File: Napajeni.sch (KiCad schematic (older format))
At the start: 8 parts, among them Q1 BS250, Q4 BS250, Q5 NTR2101P, SW2 SW_MEC_5G

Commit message: Mosfet
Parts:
- removed Q5: NTR2101P, Package_TO_SOT_SMD:SOT-23, symbol Transistor_FET:NTR2101P
- added Q2: 2N7000, Package_TO_SOT_THT:TO-92_Inline, symbol Transistor_FET:2N7000
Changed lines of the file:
@@
 	1    0    0    -1
-$EndComp
-$Comp
-L Transistor_FET:NTR2101P Q5
-U 1 1 601B9875
-P 7300 3100
-F 0 "Q5" V 7500 3050 50  0000 L CNN
-F 1 "NTR2101P" V 7500 2650 50  0000 L CNN
-F 2 "Package_TO_SOT_SMD:SOT-23" H 7500 3025 50  0001 L CIN
-F 3 "http://www.onsemi.com/pub/Collateral/NTR2101P-D.PDF" H 7300 3100 50  0001 L CNN
-	1    7300 3100
-	-1   0    0    -1
 $EndComp
 Wire Wire Line
@@
 Wire Wire Line
 	7200 2500 7200 2900
+$Comp
+L Transistor_FET:2N7000 Q2
+U 1 1 60247708
+P 7300 3100
+F 0 "Q2" H 7505 3054 50  0000 L CNN
+F 1 "2N7000" H 7505 3145 50  0000 L CNN
+F 2 "Package_TO_SOT_THT:TO-92_Inline" H 7500 3025 50  0001 L CIN
+F 3 "https://www.onsemi.com/pub/Collateral/NDS7002A-D.PDF" H 7300 3100 50  0001 L CNN
+	1    7300 3100
+	-1   0    0    1
+$EndComp
 $EndSCHEMATC

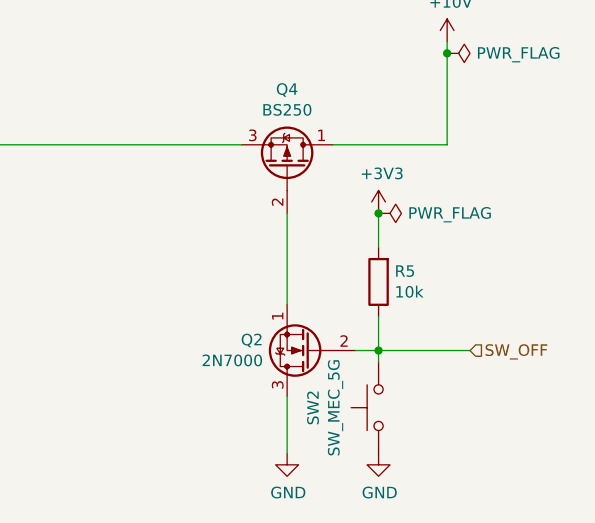
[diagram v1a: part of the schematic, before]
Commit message: Jirka upravy
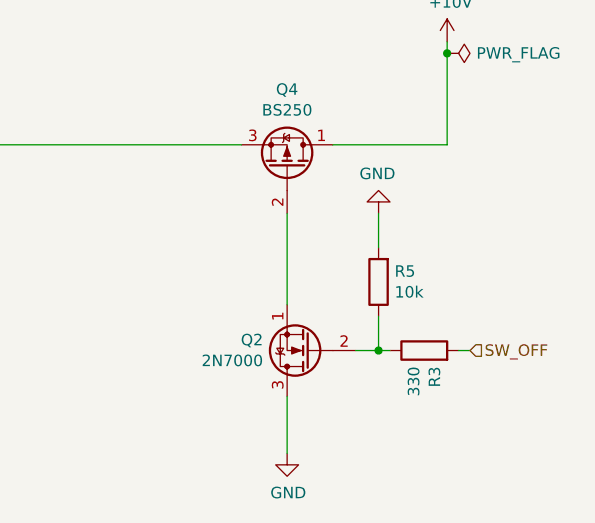
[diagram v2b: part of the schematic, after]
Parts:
- removed SW2: SW_MEC_5G, symbol Switch:SW_MEC_5G
- added R3: 330, symbol Device:R
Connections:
- net +3V3 is gone; now on net GND: R5.2
- net SW_OFF: now also R3.2; no longer Q2.2 (G), R5.1
- new net: Q2.2 (G), R3.1, R5.1
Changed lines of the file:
@@
 L power:GND #PWR011
 U 1 1 601BC6CA
-P 7600 3550
-F 0 "#PWR011" H 7600 3300 50  0001 C CNN
-F 1 "GND" H 7605 3377 50  0000 C CNN
-F 2 "" H 7600 3550 50  0001 C CNN
-F 3 "" H 7600 3550 50  0001 C CNN
-	1    7600 3550
-	1    0    0    -1
-$EndComp
-$Comp
-L Switch:SW_MEC_5G SW2
-U 1 1 601BC87E
-P 7600 3350
-F 0 "SW2" H 7600 3635 50  0000 C CNN
-F 1 "SW_MEC_5G" H 7600 3544 50  0000 C CNN
-F 2 "" H 7600 3550 50  0001 C CNN
-F 3 "http://www.apem.com/int/index.php?controller=attachment&id_attachment=488" H 7600 3550 50  0001 C CNN
-	1    7600 3350
-	0    -1   -1   0
+P 7600 2500
+F 0 "#PWR011" H 7600 2250 50  0001 C CNN
+F 1 "GND" H 7605 2327 50  0000 C CNN
+F 2 "" H 7600 2500 50  0001 C CNN
+F 3 "" H 7600 2500 50  0001 C CNN
+	1    7600 2500
+	-1   0    0    1
 $EndComp
 Wire Wire Line
 	7500 3100 7600 3100
-Wire Wire Line
-	7600 3100 7600 3150
 Wire Wire Line
 	7600 3100 7600 2950
@@
 SW_OFF
 Wire Wire Line
-	8000 3100 7600 3100
+	8000 3100 7950 3100
 $Comp
 L power:PWR_FLAG #FLG0101
@@
 Wire Wire Line
 	7600 2650 7600 2500
-$Comp
-L power:+3V3 #PWR0103
-U 1 1 601A3014
-P 7600 2500
-F 0 "#PWR0103" H 7600 2350 50  0001 C CNN
-F 1 "+3V3" H 7615 2673 50  0000 C CNN
-F 2 "" H 7600 2500 50  0001 C CNN
-F 3 "" H 7600 2500 50  0001 C CNN
-	1    7600 2500
-	1    0    0    -1
-$EndComp
-$Comp
-L power:PWR_FLAG #FLG0103
-U 1 1 601B3EBD
-P 7600 2500
-F 0 "#FLG0103" H 7600 2575 50  0001 C CNN
-F 1 "PWR_FLAG" V 7600 2628 50  0000 L CNN
-F 2 "" H 7600 2500 50  0001 C CNN
-F 3 "~" H 7600 2500 50  0001 C CNN
-	1    7600 2500
-	0    1    1    0
-$EndComp
-Connection ~ 7600 2500
 Wire Wire Line
 	4450 2500 5250 2500
@@
 	-1   0    0    1
 $EndComp
+$Comp
+L Device:R R3
+U 1 1 602489A5
+P 7800 3100
+F 0 "R3" H 7730 3054 50  0000 R CNN
+F 1 "330" H 7730 3145 50  0000 R CNN
+F 2 "" V 7730 3100 50  0001 C CNN
+F 3 "~" H 7800 3100 50  0001 C CNN
+	1    7800 3100
+	0    -1   -1   0
+$EndComp
+Wire Wire Line
+	7650 3100 7600 3100
 $EndSCHEMATC

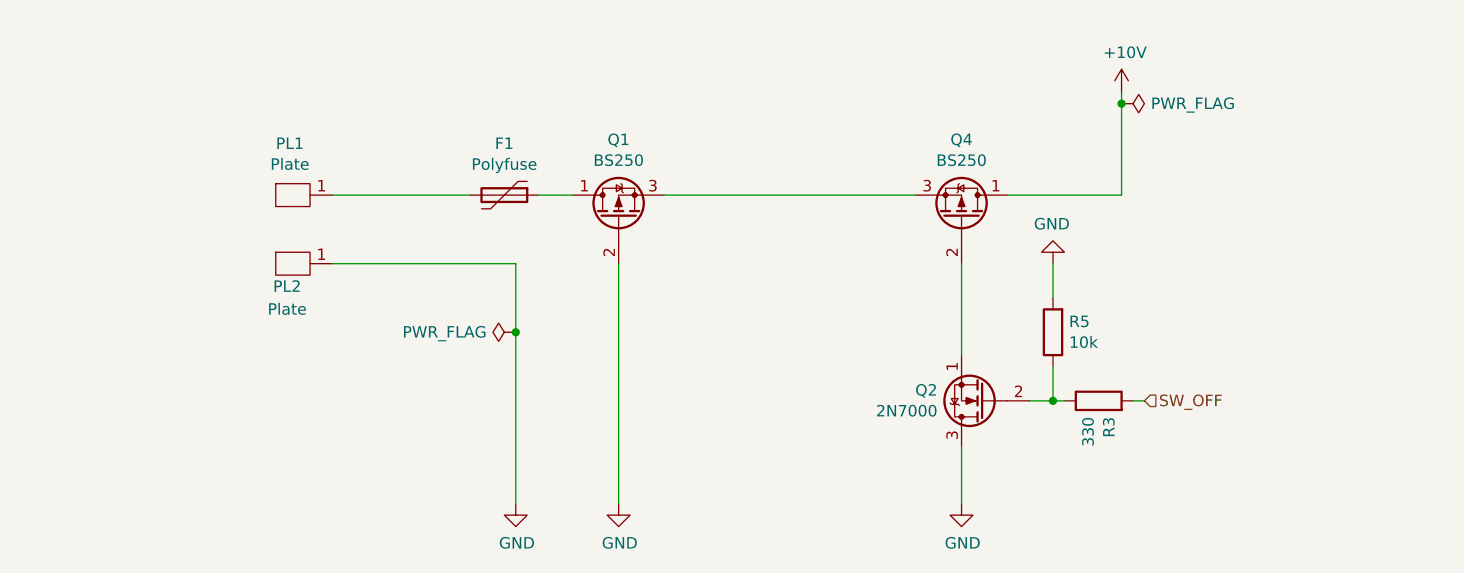
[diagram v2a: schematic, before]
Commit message: Hotové schéma
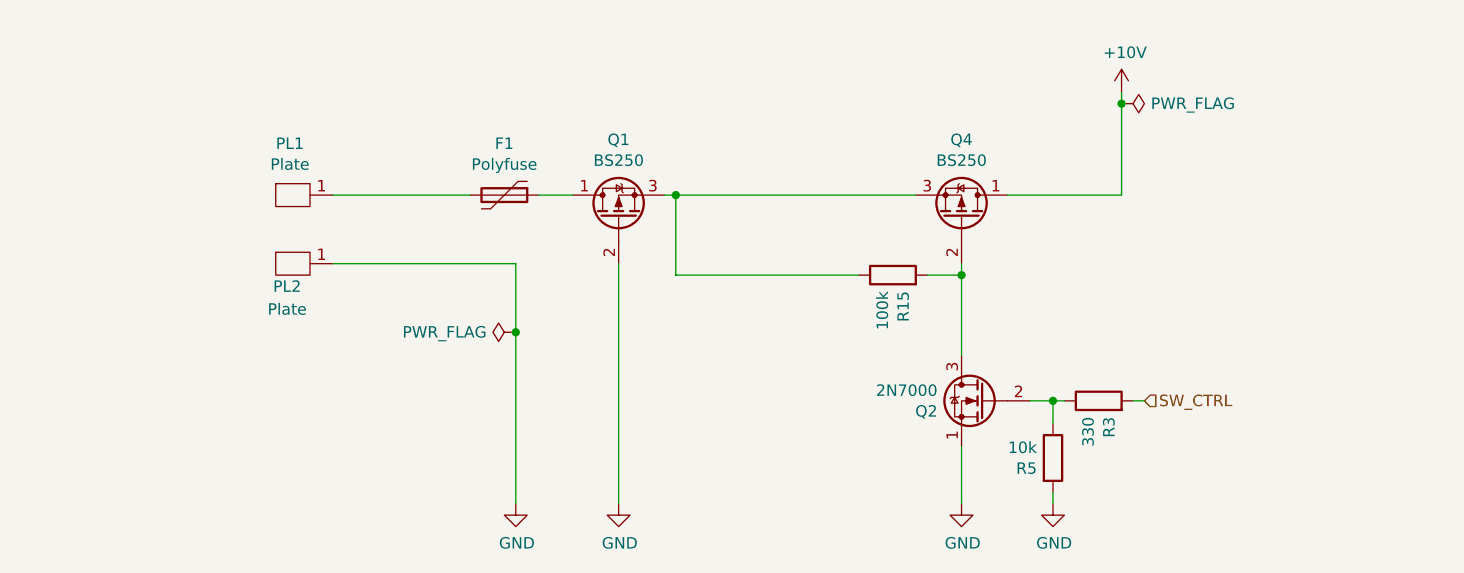
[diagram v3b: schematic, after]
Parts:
- added R15: 100k, Resistor_SMD:R_0805_2012Metric_Pad1.20x1.40mm_HandSolder, symbol Device:R
- Q2: LCSC (none) -> C8545
- R3: footprint (none) -> Resistor_SMD:R_0805_2012Metric_Pad1.20x1.40mm_HandSolder; LCSC (none) -> C17617
- R5: footprint (none) -> Resistor_SMD:R_0805_2012Metric_Pad1.20x1.40mm_HandSolder; LCSC (none) -> C17414
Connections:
- net GND: now also Q2.1 (S); no longer Q2.3 (D)
- net at Q1.3 (S), Q4.3 (S): now also R15.1
- net at Q4.2 (G): now also Q2.3 (D), R15.2; no longer Q2.1 (S)
- net SW_OFF renamed SW_CTRL
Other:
- moved on the sheet: R5
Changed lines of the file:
@@
 L Device:R R5
 U 1 1 601BBFD0
-P 7600 2800
-F 0 "R5" H 7530 2754 50  0000 R CNN
-F 1 "10k" H 7530 2845 50  0000 R CNN
-F 2 "" V 7530 2800 50  0001 C CNN
-F 3 "~" H 7600 2800 50  0001 C CNN
-	1    7600 2800
-	-1   0    0    1
+P 7600 3350
+F 0 "R5" H 7530 3304 50  0000 R CNN
+F 1 "10k" H 7530 3395 50  0000 R CNN
+F 2 "Resistor_SMD:R_0805_2012Metric_Pad1.20x1.40mm_HandSolder" V 7530 3350 50  0001 C CNN
+F 3 "~" H 7600 3350 50  0001 C CNN
+F 4 "C17414	" H 7600 3350 50  0001 C CNN "LCSC"
+	1    7600 3350
+	1    0    0    -1
 $EndComp
 $Comp
 L power:GND #PWR011
 U 1 1 601BC6CA
-P 7600 2500
-F 0 "#PWR011" H 7600 2250 50  0001 C CNN
-F 1 "GND" H 7605 2327 50  0000 C CNN
-F 2 "" H 7600 2500 50  0001 C CNN
-F 3 "" H 7600 2500 50  0001 C CNN
-	1    7600 2500
-	-1   0    0    1
+P 7600 3550
+F 0 "#PWR011" H 7600 3300 50  0001 C CNN
+F 1 "GND" H 7605 3377 50  0000 C CNN
+F 2 "" H 7600 3550 50  0001 C CNN
+F 3 "" H 7600 3550 50  0001 C CNN
+	1    7600 3550
+	1    0    0    -1
 $EndComp
-Wire Wire Line
-	7500 3100 7600 3100
-Wire Wire Line
-	7600 3100 7600 2950
-Connection ~ 7600 3100
 Text HLabel 8000 3100 2    50   Input ~ 0
-SW_OFF
+SW_CTRL
 Wire Wire Line
 	8000 3100 7950 3100
@@
 $EndComp
 Wire Wire Line
-	7600 2650 7600 2500
-Wire Wire Line
 	4450 2500 5250 2500
 $Comp
@@
 F 3 "" H 4250 2200 50  0001 C CNN
 	1    4250 2200
-	0    1    1    0
-$EndComp
-$Comp
-L Základní-deska-II-rescue:Plate-Tmc2209BreakoutBoard PL2
-U 1 1 601FAA1F
-P 4250 2500
-F 0 "PL2" V 4350 2500 50  0000 C CNN
-F 1 "Plate" V 4450 2500 50  0000 C CNN
-F 2 "" H 4250 2500 50  0001 C CNN
-F 3 "" H 4250 2500 50  0001 C CNN
-	1    4250 2500
 	0    1    1    0
 $EndComp
@@
 $EndComp
 Wire Wire Line
-	5900 2200 7000 2200
+	5900 2200 5950 2200
 Wire Wire Line
-	7200 2500 7200 2900
+	7200 2500 7200 2550
 $Comp
 L Transistor_FET:2N7000 Q2
@@
 F 2 "Package_TO_SOT_THT:TO-92_Inline" H 7500 3025 50  0001 L CIN
 F 3 "https://www.onsemi.com/pub/Collateral/NDS7002A-D.PDF" H 7300 3100 50  0001 L CNN
+F 4 "C8545" H 7300 3100 50  0001 C CNN "LCSC"
 	1    7300 3100
-	-1   0    0    1
+	-1   0    0    -1
 $EndComp
 $Comp
@@
 F 0 "R3" H 7730 3054 50  0000 R CNN
 F 1 "330" H 7730 3145 50  0000 R CNN
-F 2 "" V 7730 3100 50  0001 C CNN
+F 2 "Resistor_SMD:R_0805_2012Metric_Pad1.20x1.40mm_HandSolder" V 7730 3100 50  0001 C CNN
 F 3 "~" H 7800 3100 50  0001 C CNN
+F 4 "C17617" H 7800 3100 50  0001 C CNN "LCSC"
 	1    7800 3100
 	0    -1   -1   0
 $EndComp
+$Comp
+L Device:R R15
+U 1 1 60230BAA
+P 6900 2550
+F 0 "R15" H 6830 2504 50  0000 R CNN
+F 1 "100k" H 6830 2595 50  0000 R CNN
+F 2 "Resistor_SMD:R_0805_2012Metric_Pad1.20x1.40mm_HandSolder" V 6830 2550 50  0001 C CNN
+F 3 "~" H 6900 2550 50  0001 C CNN
+F 4 "C17407" H 6900 2550 50  0001 C CNN "LCSC"
+	1    6900 2550
+	0    -1   -1   0
+$EndComp
 Wire Wire Line
-	7650 3100 7600 3100
+	6750 2550 5950 2550
+Wire Wire Line
+	5950 2550 5950 2200
+Connection ~ 5950 2200
+Wire Wire Line
+	5950 2200 7000 2200
+Wire Wire Line
+	7050 2550 7200 2550
+Connection ~ 7200 2550
+Wire Wire Line
+	7200 2550 7200 2900
+Wire Wire Line
+	7500 3100 7600 3100
+Wire Wire Line
+	7600 3200 7600 3100
+Connection ~ 7600 3100
+Wire Wire Line
+	7600 3100 7650 3100
+Wire Wire Line
+	7600 3500 7600 3550
+$Comp
+L Základní-deska-II-rescue:Plate-Tmc2209BreakoutBoard PL2
+U 1 1 601FAA1F
+P 4250 2500
+F 0 "PL2" V 4350 2500 50  0000 C CNN
+F 1 "Plate" V 4450 2500 50  0000 C CNN
+F 2 "" H 4250 2500 50  0001 C CNN
+F 3 "" H 4250 2500 50  0001 C CNN
+	1    4250 2500
+	0    1    1    0
+$EndComp
 $EndSCHEMATC

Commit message: Hotová deska
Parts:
- F1: footprint (none) -> Fuse:Fuse_0805_2012Metric_Pad1.15x1.40mm_HandSolder
- PL1, PL2: footprint (none) -> FinalExamThesis:Plate
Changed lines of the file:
@@
 F 0 "F1" V 4975 2200 50  0000 C CNN
 F 1 "Polyfuse" V 5066 2200 50  0000 C CNN
-F 2 "" H 5250 2000 50  0001 L CNN
+F 2 "Fuse:Fuse_0805_2012Metric_Pad1.15x1.40mm_HandSolder" H 5250 2000 50  0001 L CNN
 F 3 "~" H 5200 2200 50  0001 C CNN
 	1    5200 2200
@@
 F 0 "PL1" V 4025 2212 50  0000 C CNN
 F 1 "Plate" V 4116 2212 50  0000 C CNN
-F 2 "" H 4250 2200 50  0001 C CNN
+F 2 "FinalExamThesis:Plate" H 4250 2200 50  0001 C CNN
 F 3 "" H 4250 2200 50  0001 C CNN
 	1    4250 2200
@@
 F 0 "PL2" V 4350 2500 50  0000 C CNN
 F 1 "Plate" V 4450 2500 50  0000 C CNN
-F 2 "" H 4250 2500 50  0001 C CNN
+F 2 "FinalExamThesis:Plate" H 4250 2500 50  0001 C CNN
 F 3 "" H 4250 2500 50  0001 C CNN
 	1    4250 2500

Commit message: Deska2
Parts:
- Q1, Q2, Q4: footprint Package_TO_SOT_THT:TO-92_Inline -> Package_TO_SOT_SMD:SOT-23
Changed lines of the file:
@@
 F 0 "Q4" V 7542 2300 50  0000 C CNN
 F 1 "BS250" V 7451 2300 50  0000 C CNN
-F 2 "Package_TO_SOT_THT:TO-92_Inline" H 7400 2225 50  0001 L CIN
+F 2 "Package_TO_SOT_SMD:SOT-23" H 7400 2225 50  0001 L CIN
 F 3 "http://www.vishay.com/docs/70209/70209.pdf" H 7200 2300 50  0001 L CNN
 	1    7200 2300
@@
 F 0 "Q1" V 6042 2300 50  0000 C CNN
 F 1 "BS250" V 5951 2300 50  0000 C CNN
-F 2 "Package_TO_SOT_THT:TO-92_Inline" H 5900 2225 50  0001 L CIN
+F 2 "Package_TO_SOT_SMD:SOT-23" H 5900 2225 50  0001 L CIN
 F 3 "http://www.vishay.com/docs/70209/70209.pdf" H 5700 2300 50  0001 L CNN
 	1    5700 2300
@@
 F 0 "Q2" H 7505 3054 50  0000 L CNN
 F 1 "2N7000" H 7505 3145 50  0000 L CNN
-F 2 "Package_TO_SOT_THT:TO-92_Inline" H 7500 3025 50  0001 L CIN
+F 2 "Package_TO_SOT_SMD:SOT-23" H 7500 3025 50  0001 L CIN
 F 3 "https://www.onsemi.com/pub/Collateral/NDS7002A-D.PDF" H 7300 3100 50  0001 L CNN
 F 4 "C8545" H 7300 3100 50  0001 C CNN "LCSC"

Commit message: Zmenseni desky
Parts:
- removed F1: Polyfuse, Fuse:Fuse_0805_2012Metric_Pad1.15x1.40mm_HandSolder, symbol Device:Polyfuse
- removed Q1, Q4: BS250, Package_TO_SOT_SMD:SOT-23, symbol Transistor_FET:BS250
- added iQ1, iQ2: NCE20P45Q, symbol NCE20P45Q:NCE20P45Q
- Q2: value 2N7000 -> 2N7002; symbol Transistor_FET:2N7000 -> Transistor_FET:2N7002
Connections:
- wire segments 22 -> 34
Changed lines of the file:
@@
 	1    0    0    -1
 $EndComp
-Wire Wire Line
-	5700 2500 5700 3550
-$Comp
-L Device:Polyfuse F1
-U 1 1 6019A463
-P 5200 2200
-F 0 "F1" V 4975 2200 50  0000 C CNN
-F 1 "Polyfuse" V 5066 2200 50  0000 C CNN
-F 2 "Fuse:Fuse_0805_2012Metric_Pad1.15x1.40mm_HandSolder" H 5250 2000 50  0001 L CNN
-F 3 "~" H 5200 2200 50  0001 C CNN
-	1    5200 2200
-	0    1    1    0
-$EndComp
-Wire Wire Line
-	5350 2200 5500 2200
 $Comp
 L power:GND #PWR09
@@
 Wire Wire Line
 	7200 3300 7200 3550
-Wire Wire Line
-	7400 2200 7900 2200
-Wire Wire Line
-	7900 2200 7900 1800
 $Comp
 L Device:R R5
@@
 L power:PWR_FLAG #FLG0101
 U 1 1 601A02E3
-P 7900 1800
-F 0 "#FLG0101" H 7900 1875 50  0001 C CNN
-F 1 "PWR_FLAG" V 7900 1928 50  0000 L CNN
-F 2 "" H 7900 1800 50  0001 C CNN
-F 3 "~" H 7900 1800 50  0001 C CNN
-	1    7900 1800
+P 7900 2000
+F 0 "#FLG0101" H 7900 2075 50  0001 C CNN
+F 1 "PWR_FLAG" V 7900 2128 50  0000 L CNN
+F 2 "" H 7900 2000 50  0001 C CNN
+F 3 "~" H 7900 2000 50  0001 C CNN
+	1    7900 2000
 	0    1    1    0
 $EndComp
-Connection ~ 7900 1800
-Wire Wire Line
-	7900 1800 7900 1750
 $Comp
 L power:+10V #PWR0102
@@
 Wire Wire Line
 	5250 2500 5250 2800
-Wire Wire Line
-	4450 2200 5050 2200
 $Comp
 L power:PWR_FLAG #FLG01
@@
 Wire Wire Line
 	5250 2800 5250 3550
-$Comp
-L Transistor_FET:BS250 Q4
-U 1 1 6018F4D2
-P 7200 2300
-F 0 "Q4" V 7542 2300 50  0000 C CNN
-F 1 "BS250" V 7451 2300 50  0000 C CNN
-F 2 "Package_TO_SOT_SMD:SOT-23" H 7400 2225 50  0001 L CIN
-F 3 "http://www.vishay.com/docs/70209/70209.pdf" H 7200 2300 50  0001 L CNN
-	1    7200 2300
-	0    1    -1   0
-$EndComp
-$Comp
-L Transistor_FET:BS250 Q1
-U 1 1 6018CD91
-P 5700 2300
-F 0 "Q1" V 6042 2300 50  0000 C CNN
-F 1 "BS250" V 5951 2300 50  0000 C CNN
-F 2 "Package_TO_SOT_SMD:SOT-23" H 5900 2225 50  0001 L CIN
-F 3 "http://www.vishay.com/docs/70209/70209.pdf" H 5700 2300 50  0001 L CNN
-	1    5700 2300
-	0    -1   -1   0
-$EndComp
 Wire Wire Line
 	5900 2200 5950 2200
-Wire Wire Line
-	7200 2500 7200 2550
-$Comp
-L Transistor_FET:2N7000 Q2
+$Comp
+L Transistor_FET:2N7002 Q2
 U 1 1 60247708
 P 7300 3100
 F 0 "Q2" H 7505 3054 50  0000 L CNN
-F 1 "2N7000" H 7505 3145 50  0000 L CNN
+F 1 "2N7002" H 7505 3145 50  0000 L CNN
 F 2 "Package_TO_SOT_SMD:SOT-23" H 7500 3025 50  0001 L CIN
 F 3 "https://www.onsemi.com/pub/Collateral/NDS7002A-D.PDF" H 7300 3100 50  0001 L CNN
@@
 Connection ~ 5950 2200
 Wire Wire Line
-	5950 2200 7000 2200
-Wire Wire Line
 	7050 2550 7200 2550
-Connection ~ 7200 2550
 Wire Wire Line
 	7200 2550 7200 2900
@@
 	0    1    1    0
 $EndComp
+$Comp
+L NCE20P45Q:NCE20P45Q iQ1
+U 1 1 602FAA88
+P 5650 2250
+F 0 "iQ1" H 5650 2625 50  0000 C CNN
+F 1 "NCE20P45Q" H 5650 2534 50  0000 C CNN
+F 2 "" H 5550 2350 50  0001 C CNN
+F 3 "" H 5550 2350 50  0001 C CNN
+	1    5650 2250
+	1    0    0    -1
+$EndComp
+Wire Wire Line
+	5900 2400 5900 2300
+Wire Wire Line
+	5900 2300 5900 2200
+Connection ~ 5900 2300
+Connection ~ 5900 2200
+Wire Wire Line
+	5900 2200 5900 2100
+Wire Wire Line
+	5400 2300 5400 2200
+Connection ~ 5400 2200
+Wire Wire Line
+	5400 2100 5400 2200
+Wire Wire Line
+	5400 2400 5400 2650
+Wire Wire Line
+	5400 2650 5700 2650
+Wire Wire Line
+	5700 2650 5700 3550
+Wire Wire Line
+	5950 2200 7000 2200
+$Comp
+L NCE20P45Q:NCE20P45Q iQ2
+U 1 1 60300EC1
+P 7250 2250
+F 0 "iQ2" H 7250 2625 50  0000 C CNN
+F 1 "NCE20P45Q" H 7250 2534 50  0000 C CNN
+F 2 "" H 7150 2350 50  0001 C CNN
+F 3 "" H 7150 2350 50  0001 C CNN
+	1    7250 2250
+	-1   0    0    -1
+$EndComp
+Wire Wire Line
+	7000 2400 7000 2300
+Connection ~ 7000 2200
+Wire Wire Line
+	7000 2200 7000 2100
+Connection ~ 7000 2300
+Wire Wire Line
+	7000 2300 7000 2200
+Wire Wire Line
+	7500 2100 7500 2200
+Connection ~ 7500 2200
+Wire Wire Line
+	7500 2200 7500 2300
+Wire Wire Line
+	7500 2200 7900 2200
+Wire Wire Line
+	7200 2550 7500 2550
+Wire Wire Line
+	7500 2550 7500 2400
+Connection ~ 7200 2550
+Wire Wire Line
+	7900 1750 7900 2000
+Connection ~ 7900 2000
+Wire Wire Line
+	7900 2000 7900 2200
+Wire Wire Line
+	4450 2200 5400 2200
 $EndSCHEMATC

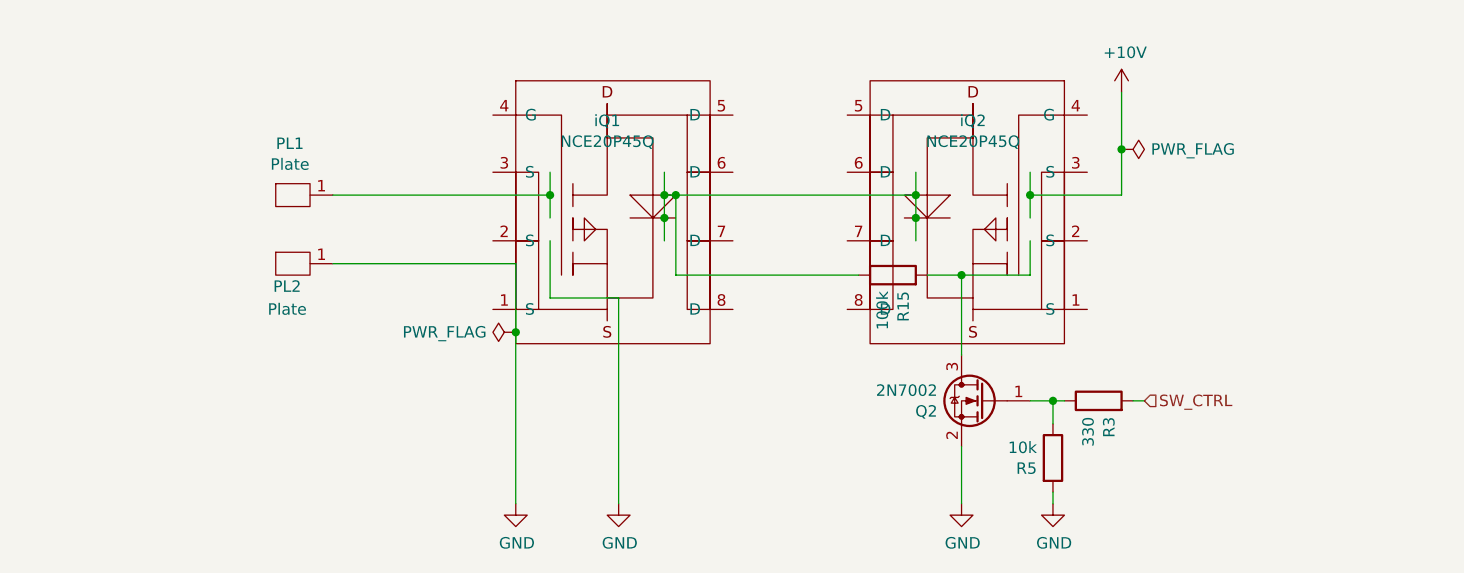
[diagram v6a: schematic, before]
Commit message: Jirka
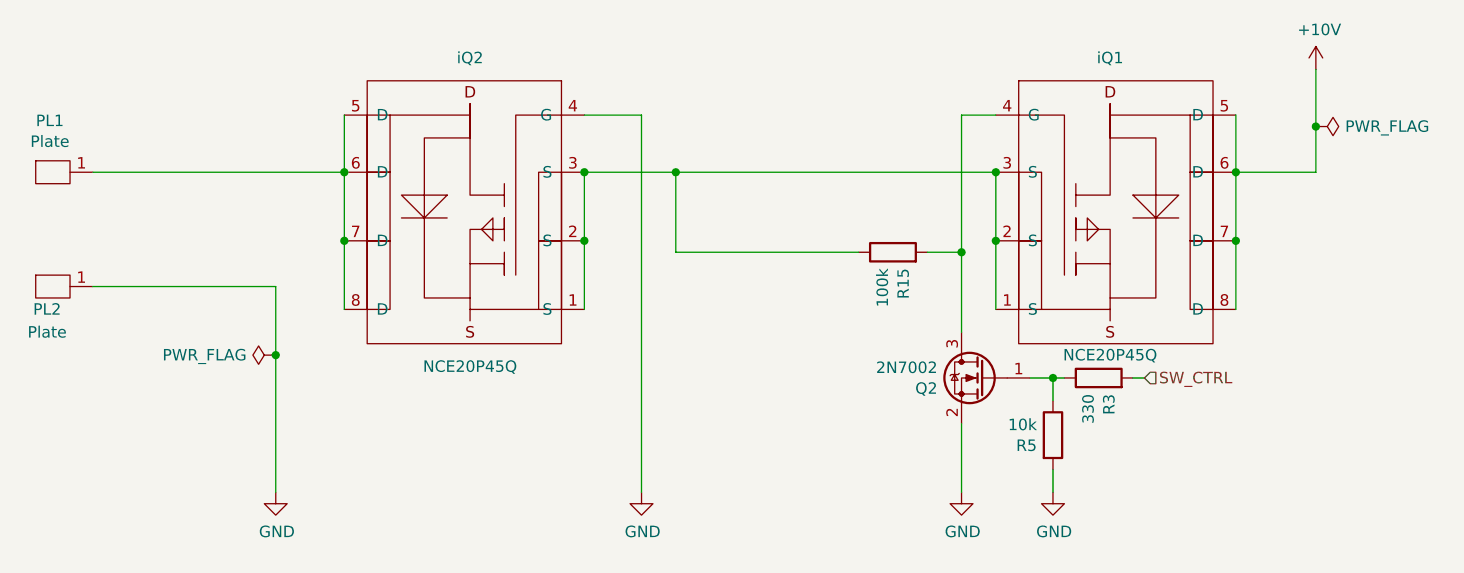
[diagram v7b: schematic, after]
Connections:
- wire segments 34 -> 33
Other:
- moved on the sheet: PL1, PL2, Q2, R15, R3, R5, iQ1, iQ2
